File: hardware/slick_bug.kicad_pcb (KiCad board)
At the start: 2 copper layers, 20.2 x 23.1 mm, 10 parts, among them J1 Conn_01x04_Socket, J2 Conn_01x04_Socket, U1 XIAO-RP2040-SMD, U4 MAX40203AUK+T

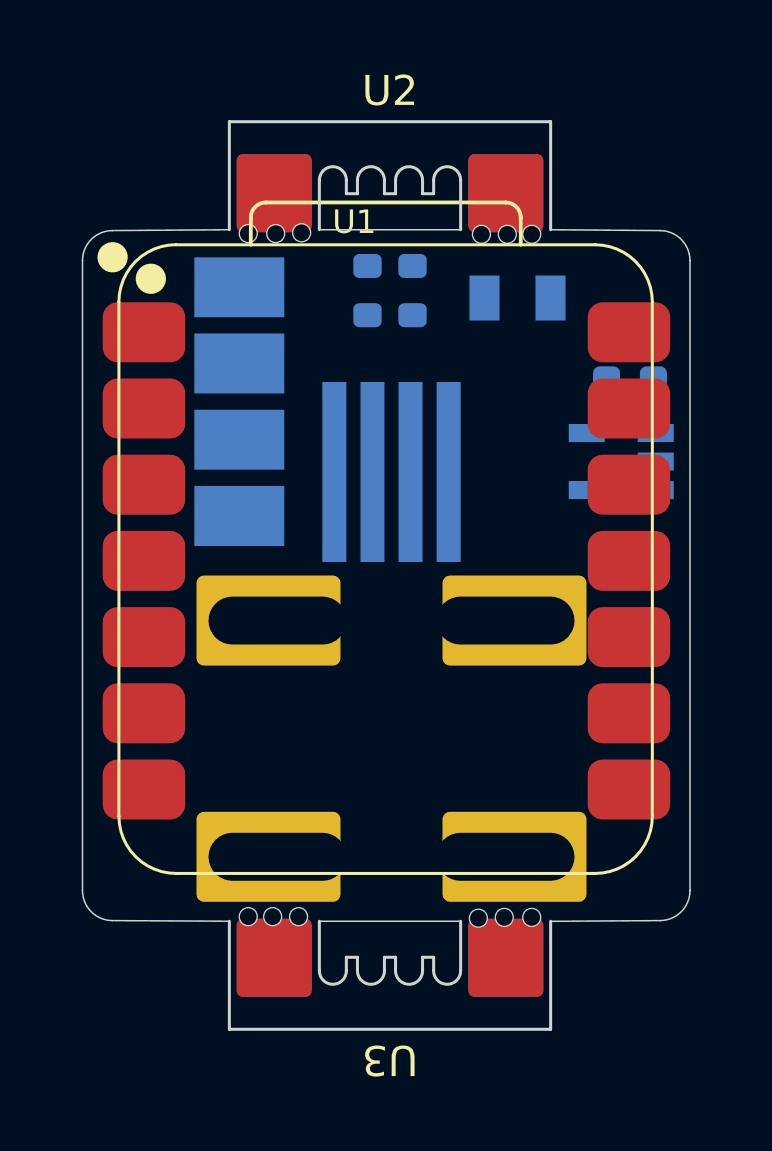
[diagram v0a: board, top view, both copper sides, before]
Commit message: pin order change
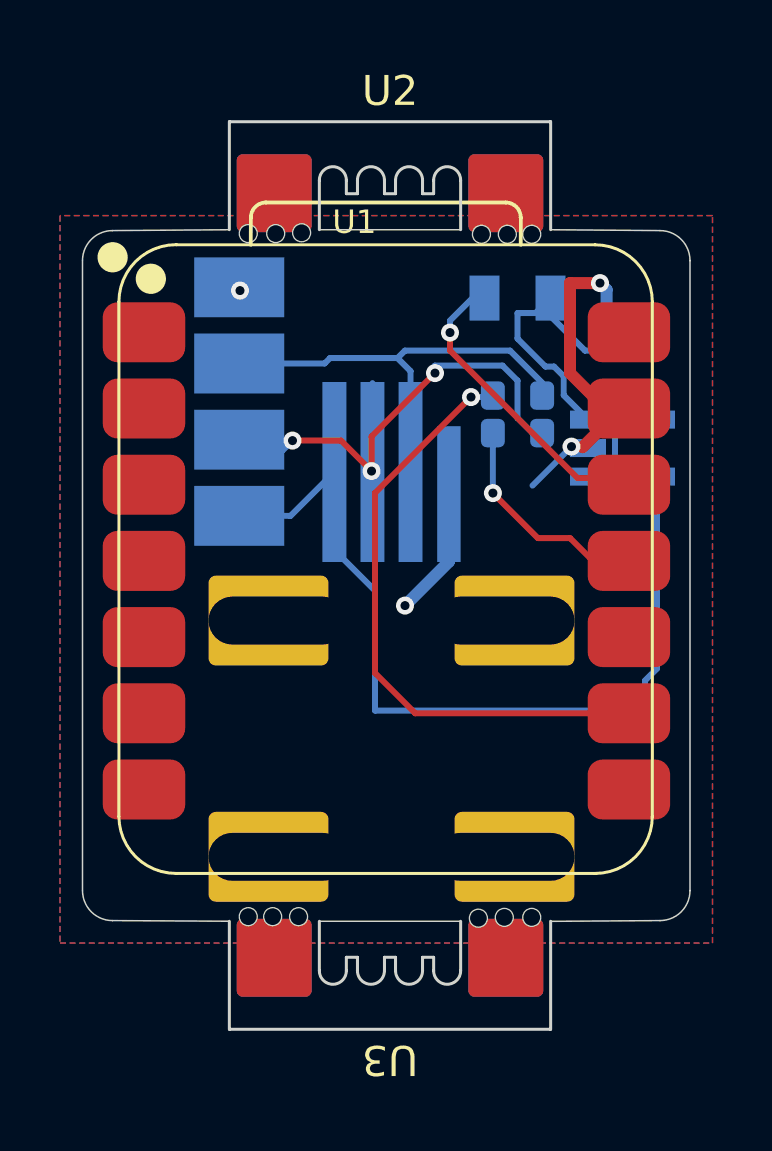
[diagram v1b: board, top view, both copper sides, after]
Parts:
- moved R2 6.10 mm to (95.0, 65.5), turned to 0 degrees
- moved R1 5.90 mm to (95.0, 66.8), turned to 0 degrees
- moved C1 2.00 mm to (98.8, 63.0)
- moved U4 0.45 mm to (98.5, 67.2), turned to 180 degrees
- turned F1 to 0 degrees
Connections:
- J1 pad 1: TARGET_VCC -> GND
- J1 pad 2: TARGET_SWDIO -> TARGET_SWCLK
- J1 pad 3: TARGET_SWCLK -> TARGET_SWDIO
- J1 pad 4: GND -> TARGET_VCC
- J2 pad 1: TARGET_VCC -> GND
- J2 pad 2: TARGET_SWDIO -> TARGET_SWCLK
- J2 pad 3: TARGET_SWCLK -> TARGET_SWDIO
- J2 pad 4: GND -> TARGET_VCC
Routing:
- net TARGET_VCC: track 0.00 -> 29.3 mm
- net Net-(U1-D8): track 0.00 -> 20.3 mm, vias 0 -> 1
- net GND: track 0.00 -> 17.3 mm, vias 0 -> 4
- net TARGET_SWDIO: track 0.00 -> 17.0 mm, vias 0 -> 3
- net TARGET_SWCLK: track 0.00 -> 15.1 mm
- net Net-(U4-EN): track 0.00 -> 15.0 mm
- net Net-(U1-3V3_OUT): track 0.00 -> 10.3 mm, vias 0 -> 1
- net Net-(U1-D10): track 0.00 -> 7.47 mm, vias 0 -> 1
- added copper zone on B.Cu, net GND
- added copper zone on F.Cu, net GND
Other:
- board text added: "DIO"
- board text removed: "IO"

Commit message: slick bug
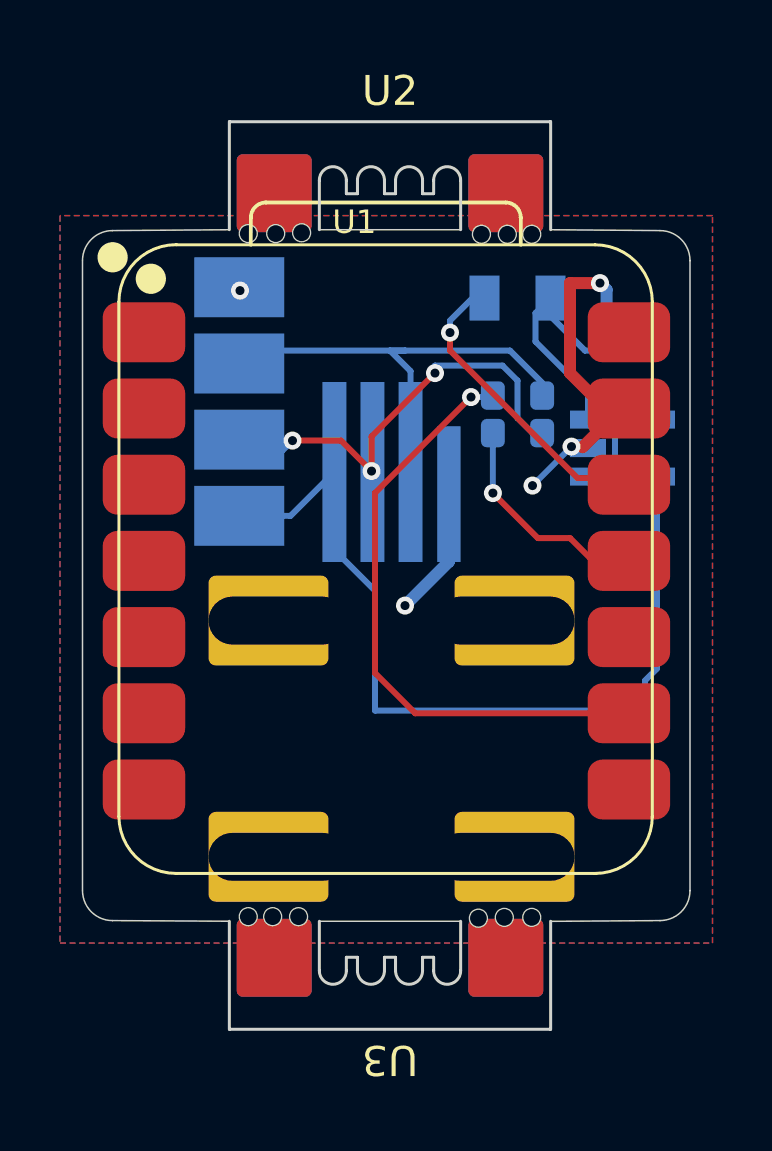
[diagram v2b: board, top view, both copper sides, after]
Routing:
- net TARGET_SWDIO: track 17.0 -> 14.1 mm
- net TARGET_VCC: track 29.3 -> 26.7 mm
- net Net-(U4-EN): track 15.0 -> 12.7 mm
- net GND: track 17.3 -> 15.7 mm, vias 4 -> 5
- net Net-(U1-D10): track 7.47 -> 6.27 mm
- net TARGET_SWCLK: track 15.1 -> 16.0 mm
- net Net-(U1-3V3_OUT): track 10.3 -> 9.56 mm
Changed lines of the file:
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@@
 			)
 		)
-		(attr through_hole)
+		(attr through_hole exclude_from_bom)
 		(duplicate_pad_numbers_are_jumpers no)
 		(fp_line
@@
 			)
 		)
-		(attr through_hole)
+		(attr through_hole exclude_from_bom)
 		(duplicate_pad_numbers_are_jumpers no)
 		(fp_line
@@
 			)
 		)
+		(attr exclude_from_bom)
 		(duplicate_pad_numbers_are_jumpers no)
 		(fp_line
@@
 			)
 		)
-		(property "Description" ""
+		(property "Description" "Generic connector, single row, 01x04, script generated"
 			(at 0 0 0)
 			(unlocked yes)
@@
 		(sheetname "/")
 		(sheetfile "slick_bug.kicad_sch")
-		(attr through_hole)
+		(units
+			(unit
+				(name "A")
+				(pins "1" "2" "3" "4")
+			)
+		)
+		(attr through_hole exclude_from_bom)
 		(duplicate_pad_numbers_are_jumpers no)
 		(fp_line
@@
 			)
 		)
-		(attr smd)
+		(attr smd exclude_from_bom)
 		(duplicate_pad_numbers_are_jumpers no)
 		(fp_line
@@
 	)
 	(segment
-		(start 94.130735 65.549265)
-		(end 94.18 65.5)
-		(width 0.2)
-		(layer "B.Cu")
-		(net "Net-(U1-D8)")
-	)
-	(segment
 		(start 93.450735 65.549265)
 		(end 94.130735 65.549265)
@@
 	)
 	(segment
-		(start 97.5105 71.0105)
-		(end 98.714 71.0105)
-		(width 0.2)
-		(layer "F.Cu")
-		(net "Net-(U1-D10)")
-	)
-	(segment
 		(start 94.18 68.75)
 		(end 95.68 70.25)
@@
 	)
 	(segment
-		(start 98.4935 68.25)
-		(end 98.714 68.4705)
-		(width 0.2)
-		(layer "F.Cu")
-		(net "Net-(U1-3V3_OUT)")
-	)
-	(segment
 		(start 92.75 63.4)
 		(end 92.75 64)
@@
 	)
 	(segment
-		(start 93.5 62.25)
-		(end 93.9 62.25)
-		(width 0.2)
-		(layer "B.Cu")
-		(net "Net-(U1-3V3_OUT)")
-	)
-	(segment
 		(start 92.75 63.4)
 		(end 92.75 63)
@@
 		(net "GND")
 	)
-	(segment
-		(start 98.714 65.9305)
-		(end 98.461963 65.9305)
-		(width 0.4)
-		(layer "F.Cu")
-		(net "GND")
-	)
-	(segment
-		(start 98.714 65.9305)
-		(end 97.9305 65.9305)
-		(width 0.4)
-		(layer "F.Cu")
-		(net "GND")
-	)
 	(via
 		(at 85.75 62)
@@
 		(net "GND")
 	)
-	(segment
-		(start 96.84853 67.25)
-		(end 96.799265 67.200735)
-		(width 0.2)
-		(layer "B.Cu")
+	(via
+		(at 95.5 68.5)
+		(size 0.6)
+		(drill 0.3)
+		(layers "F.Cu" "B.Cu")
 		(net "GND")
 	)
 	(segment
-		(start 96.799265 67.200735)
-		(end 95.5 68.5)
+		(start 96.84853 67.25)
+		(end 96.799265 67.200735)
 		(width 0.2)
 		(layer "B.Cu")
@@
 	)
 	(segment
-		(start 97.35 67.25)
-		(end 96.84853 67.25)
+		(start 95.5 68.5)
+		(end 96.799265 67.200735)
 		(width 0.2)
 		(layer "B.Cu")
@@
 	)
 	(segment
-		(start 85.725 61.89)
-		(end 85.725 61.975)
-		(width 0.4)
-		(layer "B.Cu")
-		(net "GND")
-	)
-	(segment
-		(start 85.725 61.975)
-		(end 85.75 62)
-		(width 0.4)
-		(layer "B.Cu")
-		(net "GND")
-	)
-	(segment
 		(start 92.7145 68.785)
 		(end 92.7145 71.0355)
@@
 	)
 	(segment
-		(start 95.82 65.07)
-		(end 94.75 64)
-		(width 0.2)
-		(layer "B.Cu")
-		(net "TARGET_SWCLK")
-	)
-	(segment
-		(start 91.435 64.685)
-		(end 91.435 68.047)
+		(start 85.725 64.43)
+		(end 86.155 64)
 		(width 0.2)
 		(layer "B.Cu")
@@
 	)
 	(segment
-		(start 88.57 64.43)
-		(end 88.75 64.25)
+		(start 95.82 65.07)
+		(end 94.75 64)
 		(width 0.2)
 		(layer "B.Cu")
@@
 	)
 	(segment
-		(start 88.75 64.25)
-		(end 91 64.25)
+		(start 86.155 64)
+		(end 91.25 64)
 		(width 0.2)
 		(layer "B.Cu")
@@
 	)
 	(segment
-		(start 91 64.25)
+		(start 90.75 64)
 		(end 91.435 64.685)
 		(width 0.2)
@@
 	)
 	(segment
-		(start 85.725 64.43)
-		(end 88.57 64.43)
+		(start 91.435 64.685)
+		(end 91.435 68.047)
 		(width 0.2)
 		(layer "B.Cu")
@@
 	)
 	(segment
-		(start 91.25 64)
-		(end 91 64.25)
+		(start 95.82 65.5)
+		(end 95.82 65.07)
 		(width 0.2)
 		(layer "B.Cu")
@@
 	)
 	(segment
-		(start 95.82 65.5)
-		(end 95.82 65.07)
+		(start 91.25 64)
+		(end 90.75 64)
 		(width 0.2)
 		(layer "B.Cu")
@@
 	)
 	(segment
-		(start 96.540346 65.490346)
-		(end 97.35 66.3)
-		(width 0.2)
-		(layer "B.Cu")
-		(net "Net-(U4-EN)")
-	)
-	(segment
-		(start 96.217157 64.532843)
-		(end 95.934314 64.532843)
-		(width 0.2)
-		(layer "B.Cu")
-		(net "Net-(U4-EN)")
-	)
-	(segment
 		(start 99.53 63)
 		(end 98.53 64)
@@
 	)
 	(segment
-		(start 95 63.598529)
-		(end 95 62.75)
-		(width 0.2)
-		(layer "B.Cu")
-		(net "Net-(U4-EN)")
-	)
-	(segment
-		(start 96.540346 64.856032)
-		(end 96.217157 64.532843)
+		(start 95.6 62.75)
+		(end 96.1 62.25)
 		(width 0.2)
 		(layer "B.Cu")
@@
 	)
 	(segment
-		(start 95.6 62.75)
-		(end 96.1 62.25)
+		(start 97.35 66.3)
+		(end 97.35 65.45)
 		(width 0.2)
 		(layer "B.Cu")
@@
 	)
 	(segment
-		(start 96.1 62.25)
-		(end 96.1 62.85)
+		(start 95.6 63.7)
+		(end 95.6 62.75)
 		(width 0.2)
 		(layer "B.Cu")
@@
 	)
 	(segment
-		(start 96.540346 65.490346)
-		(end 96.540346 64.856032)
-		(width 0.2)
-		(layer "B.Cu")
-		(net "Net-(U4-EN)")
-	)
-	(segment
 		(start 98.15 66.3)
 		(end 97.35 66.3)
@@
 	)
 	(segment
-		(start 95.934314 64.532843)
-		(end 95 63.598529)
-		(width 0.2)
-		(layer "B.Cu")
-		(net "Net-(U4-EN)")
-	)
-	(segment
 		(start 97.35 68.2)
 		(end 97.9 68.2)
@@
 	)
 	(segment
-		(start 96.1 62.25)
-		(end 96.78 62.25)
-		(width 0.2)
-		(layer "B.Cu")
-		(net "Net-(U4-EN)")
-	)
-	(segment
-		(start 95 62.75)
-		(end 95.6 62.75)
+		(start 97.35 65.45)
+		(end 95.6 63.7)
 		(width 0.2)
 		(layer "B.Cu")
@@
 	)
 	(segment
-		(start 88.895 68.047)
-		(end 88.895 70.647)
-		(width 0.2)
-		(layer "B.Cu")
-		(net "TARGET_VCC")
-	)
-	(segment
 		(start 99.25 76)
 		(end 99.25 75)
@@
 	)
 	(segment
-		(start 85.74 69.51)
-		(end 85.75 69.5)
-		(width 0.2)
-		(layer "B.Cu")
-		(net "TARGET_VCC")
-	)
-	(segment
 		(start 87.432 69.51)
 		(end 88.895 68.047)
@@
 	)
 	(segment
-		(start 85.725 69.51)
-		(end 85.74 69.51)
-		(width 0.2)
-		(layer "B.Cu")
-		(net "TARGET_VCC")
-	)
-	(segment
 		(start 99.65 74.6)
 		(end 99.65 68.2)
@@
 		(width 0.2)
 		(layer "B.Cu")
-		(net "TARGET_SWDIO")
-	)
-	(segment
-		(start 90.165 65.085)
-		(end 90.165 68.047)
-		(width 0.2)
-		(layer "B.Cu")
